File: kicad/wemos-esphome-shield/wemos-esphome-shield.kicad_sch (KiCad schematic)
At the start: 24 parts, among them Q1 2N2219, Q2 2N2219, Q3 2N2219, T1 Transformer_1P_1S, U2 WeMos_D1_mini

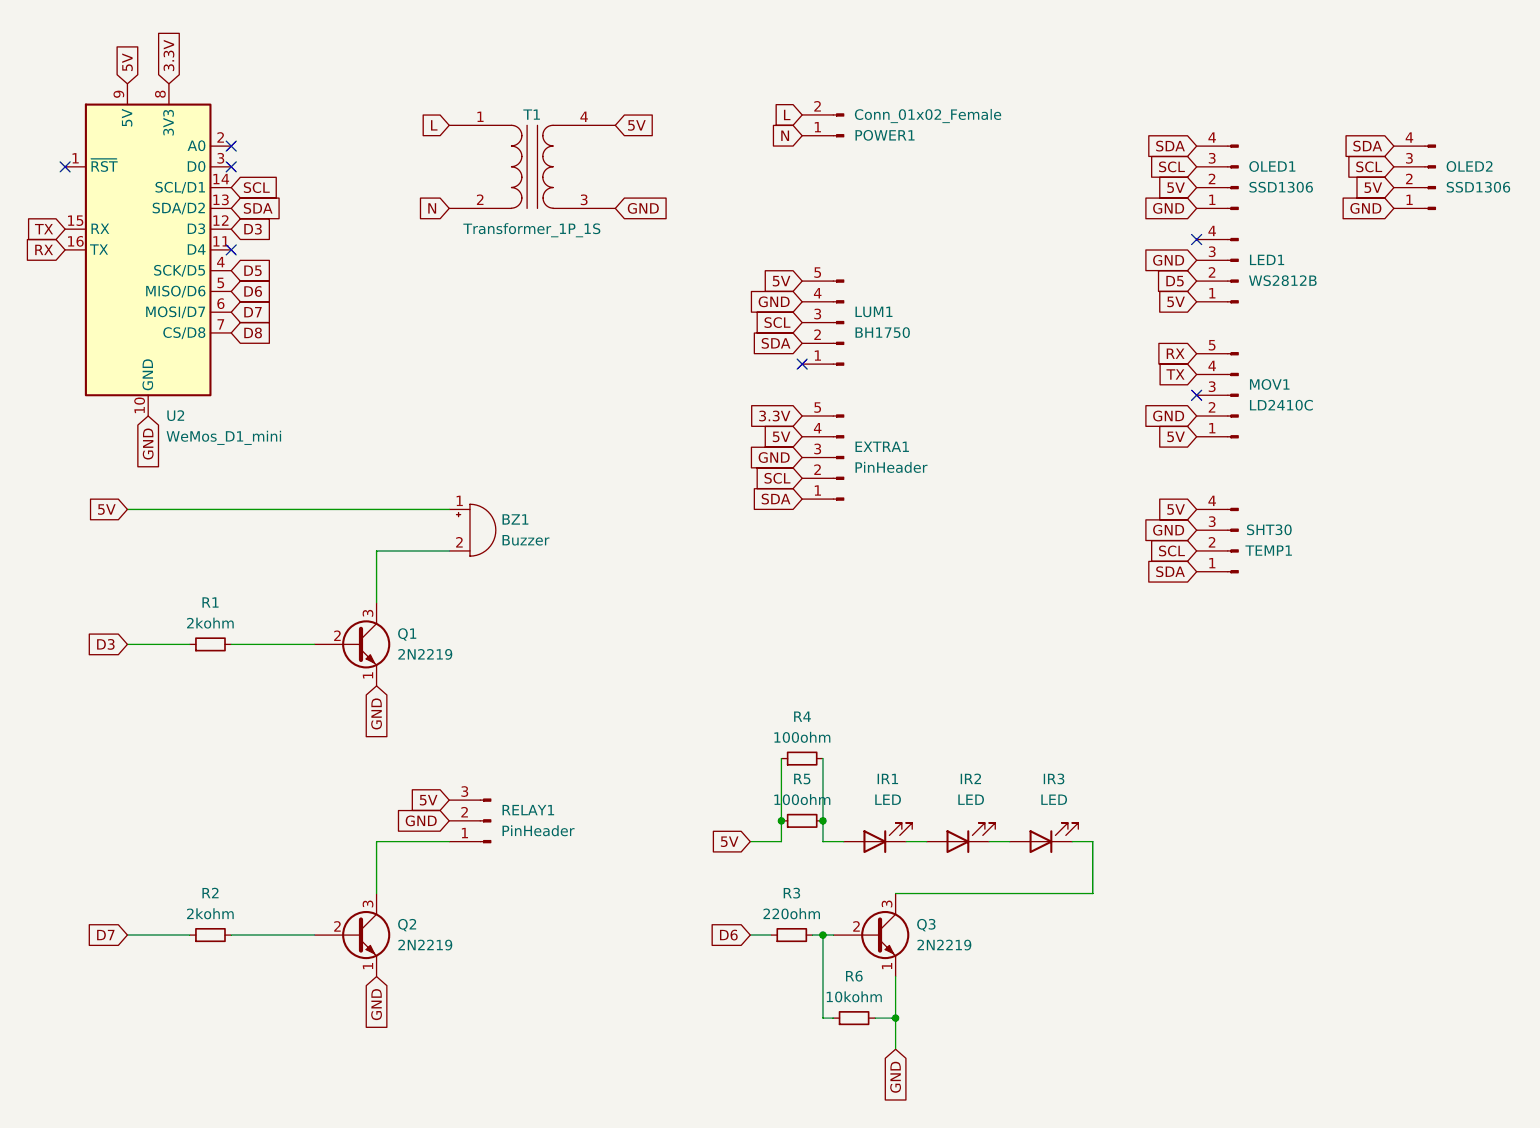
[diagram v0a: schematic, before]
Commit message: update schematics
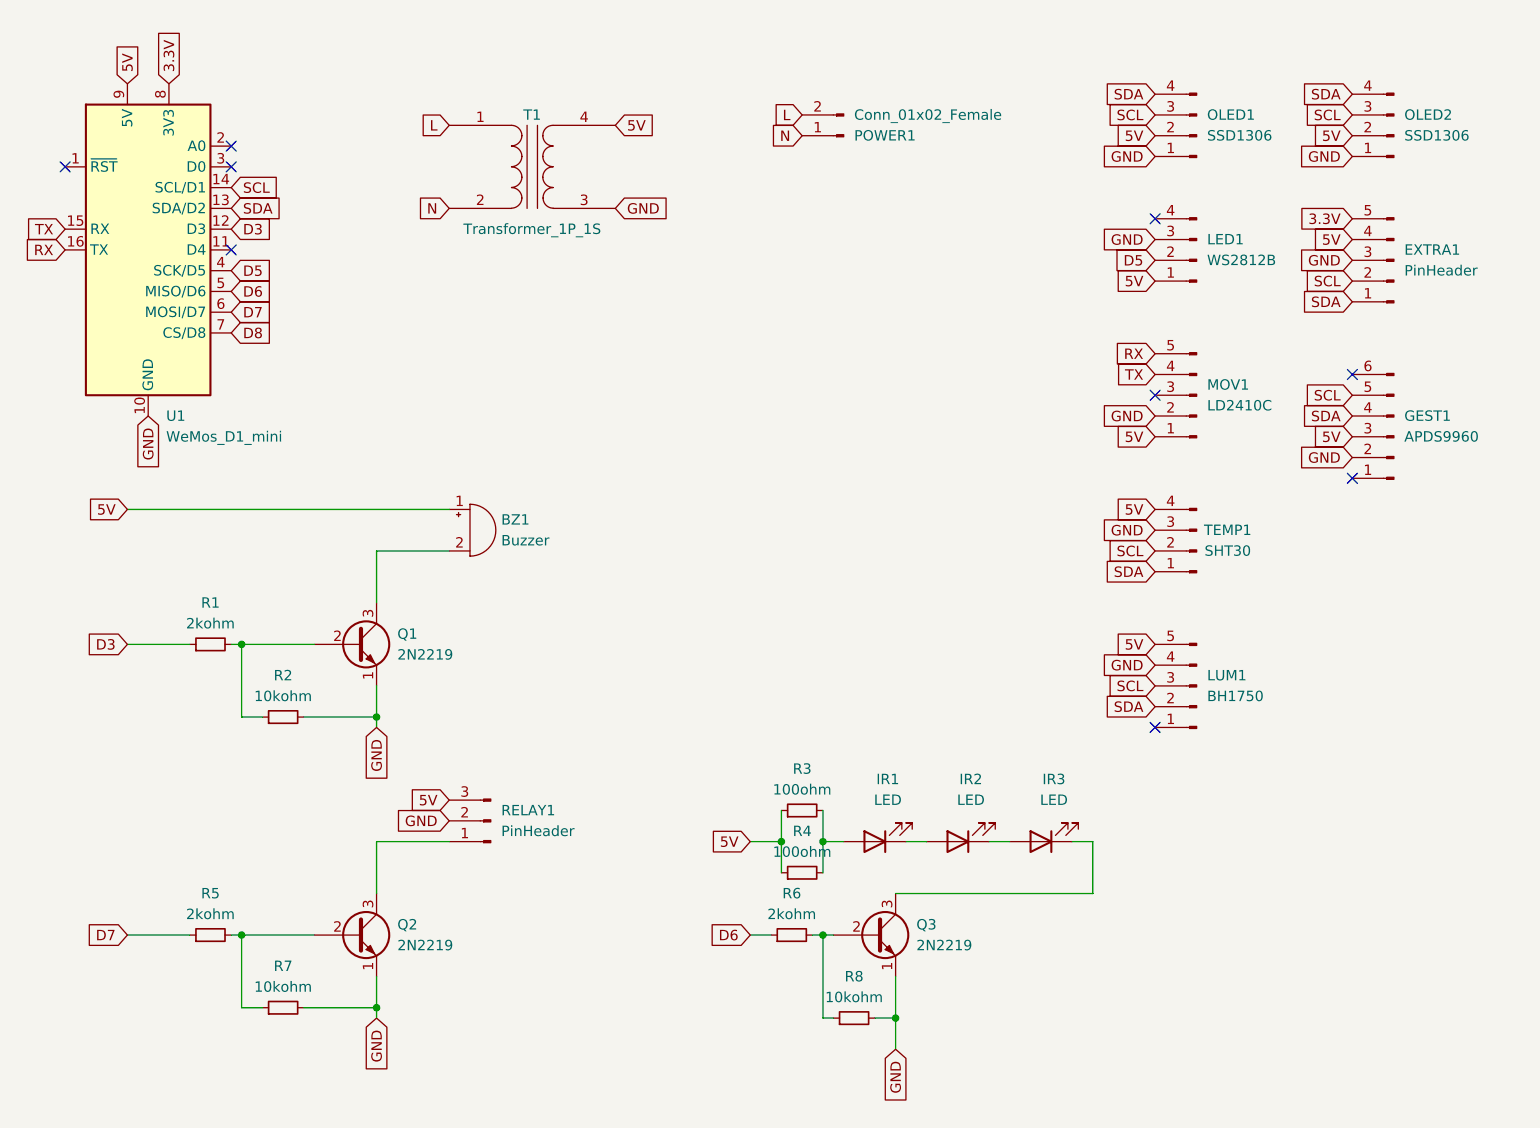
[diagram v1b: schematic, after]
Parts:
- added GEST1: APDS9960, symbol Connector:Conn_01x06_Pin
- added R2, R7: 10kohm, symbol Device:R_Small
- R6: renamed from R3; value 220ohm -> 2kohm
- renumbered R4 to R3, R5 to R4, R2 to R5, R6 to R8, U2 to U1
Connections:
- net 5V: now also GEST1.3 (Pin_3)
- net GND: now also GEST1.2 (Pin_2), R2.2, R7.2
- net SCL: now also GEST1.5 (Pin_5)
- net SDA: now also GEST1.4 (Pin_4)
- net at Q2.2 (B), R5.2: now also R7.1
- net at Q1.2 (B), R1.2: now also R2.1
- no-connect marks 7 -> 9
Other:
- moved on the sheet: EXTRA1, LED1, LUM1, MOV1, OLED1, OLED2, R3, R4, TEMP1
